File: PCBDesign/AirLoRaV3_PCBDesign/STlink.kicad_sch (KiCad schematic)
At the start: 1 part, among them J7 UART2

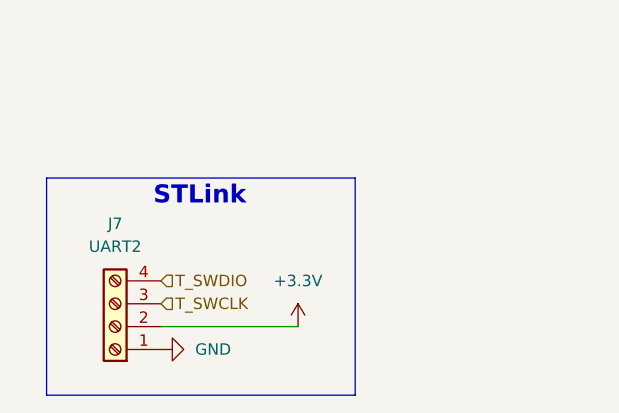
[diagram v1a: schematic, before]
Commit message: Update schematic
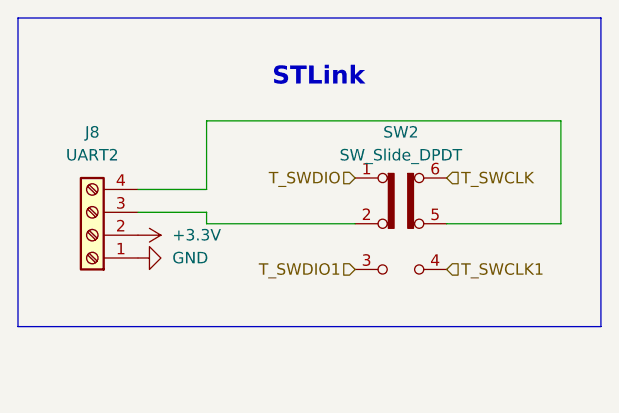
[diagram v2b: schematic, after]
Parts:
- added SW2: SW_Slide_DPDT, Button_Switch_THT:SW_E-Switch_EG1271_SPDT, symbol Switch:SW_Slide_DPDT
- renumbered J7 to J8
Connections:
- net T_SWCLK: now also SW2.6 (C); no longer J8.3 (Pin_3)
- net T_SWDIO: now also SW2.1 (A); no longer J8.4 (Pin_4)
- new net: J8.3 (Pin_3), SW2.2 (B)
- new net: J8.4 (Pin_4), SW2.5 (B)
- new net T_SWCLK1: SW2.4 (A)
- new net T_SWDIO1: SW2.3 (C)
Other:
- moved on the sheet: J8
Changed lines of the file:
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@@
 	(wire
 		(pts
-			(xy 142.24 100.33) (xy 157.48 100.33)
+			(xy 147.32 77.47) (xy 147.32 85.09)
+		)
+		(stroke
+			(width 0)
+			(type default)
+		)
+	)
+	(wire
+		(pts
+			(xy 147.32 85.09) (xy 139.7 85.09)
+		)
+		(stroke
+			(width 0)
+			(type default)
+		)
+	)
+	(wire
+		(pts
+			(xy 147.32 88.9) (xy 163.83 88.9)
+		)
+		(stroke
+			(width 0)
+			(type default)
+		)
+	)
+	(wire
+		(pts
+			(xy 147.32 87.63) (xy 139.7 87.63)
+		)
+		(stroke
+			(width 0)
+			(type default)
+		)
+	)
+	(wire
+		(pts
+			(xy 186.69 88.9) (xy 186.69 77.47)
+		)
+		(stroke
+			(width 0)
+			(type default)
+		)
+	)
+	(wire
+		(pts
+			(xy 186.69 77.47) (xy 147.32 77.47)
+		)
+		(stroke
+			(width 0)
+			(type default)
+		)
+	)
+	(wire
+		(pts
+			(xy 147.32 88.9) (xy 147.32 87.63)
+		)
+		(stroke
+			(width 0)
+			(type default)
+		)
+	)
+	(wire
+		(pts
+			(xy 173.99 88.9) (xy 186.69 88.9)
 		)
 		(stroke
@@
 	)
 	(rectangle
-		(start 129.54 83.82)
-		(end 163.83 107.95)
+		(start 126.365 66.04)
+		(end 191.135 100.33)
 		(stroke
 			(width 0)
@@
 	(text "STLink"
 		(exclude_from_sim no)
-		(at 146.558 85.852 0)
+		(at 159.766 72.644 0)
 		(effects
 			(font
@@
 		)
 	)
-	(hierarchical_label "T_SWCLK"
+	(hierarchical_label "T_SWCLK1"
 		(shape input)
-		(at 142.24 97.79 0)
+		(at 173.99 93.98 0)
 		(fields_autoplaced yes)
 		(effects
@@
 		)
 	)
-	(hierarchical_label "T_SWDIO"
+	(hierarchical_label "T_SWCLK"
 		(shape input)
-		(at 142.24 95.25 0)
+		(at 173.99 83.82 0)
 		(fields_autoplaced yes)
 		(effects
@@
 		)
 	)
+	(hierarchical_label "T_SWDIO"
+		(shape input)
+		(at 163.83 83.82 180)
+		(fields_autoplaced yes)
+		(effects
+			(font
+				(size 1.27 1.27)
+			)
+			(justify right)
+		)
+	)
+	(hierarchical_label "T_SWDIO1"
+		(shape input)
+		(at 163.83 93.98 180)
+		(fields_autoplaced yes)
+		(effects
+			(font
+				(size 1.27 1.27)
+			)
+			(justify right)
+		)
+	)
 	(symbol
 		(lib_id "Connector:Screw_Terminal_01x04")
-		(at 137.16 100.33 180)
+		(at 134.62 90.17 180)
 		(unit 1)
 		(exclude_from_sim no)
@@
 		(dnp no)
 		(fields_autoplaced yes)
-		(property "Reference" "J7"
-			(at 137.16 88.9 0)
+		(property "Reference" "J8"
+			(at 134.62 78.74 0)
 			(effects
 				(font
@@
 		)
 		(property "Value" "UART2"
-			(at 137.16 91.44 0)
+			(at 134.62 81.28 0)
 			(effects
 				(font
@@
 		)
 		(property "Footprint" "Connector_JST:JST_XH_B4B-XH-A_1x04_P2.50mm_Vertical"
-			(at 137.16 100.33 0)
+			(at 134.62 90.17 0)
 			(effects
 				(font
@@
 		)
 		(property "Datasheet" "~"
-			(at 137.16 100.33 0)
+			(at 134.62 90.17 0)
 			(effects
 				(font
@@
 		)
 		(property "Description" ""
-			(at 137.16 100.33 0)
+			(at 134.62 90.17 0)
 			(effects
 				(font
@@
 		)
 		(property "MANUFACTURER" ""
-			(at 137.16 100.33 0)
+			(at 134.62 90.17 0)
 			(effects
 				(font
@@
 		)
 		(property "MAXIMUM_PACKAGE_HEIGHT" ""
-			(at 137.16 100.33 0)
+			(at 134.62 90.17 0)
 			(effects
 				(font
@@
 		)
 		(property "PARTREV" ""
-			(at 137.16 100.33 0)
+			(at 134.62 90.17 0)
 			(effects
 				(font
@@
 		)
 		(property "STANDARD" ""
-			(at 137.16 100.33 0)
+			(at 134.62 90.17 0)
 			(effects
 				(font
@@
 			(project "airlora-kicad"
 				(path "/59d971df-d6c1-4ef7-a085-bf08b7b16047/be77b740-d58b-414b-97ce-61f1d1685314/0fe76900-3fef-41a8-aa6f-27268a6f6f64"
-					(reference "J7")
+					(reference "J8")
 					(unit 1)
 				)
@@
 	(symbol
 		(lib_id "power:GND")
-		(at 142.24 102.87 90)
+		(at 139.7 92.71 90)
 		(unit 1)
 		(exclude_from_sim no)
@@
 		(dnp no)
 		(fields_autoplaced yes)
-		(property "Reference" "#PWR043"
-			(at 148.59 102.87 0)
+		(property "Reference" "#PWR046"
+			(at 146.05 92.71 0)
 			(effects
 				(font
@@
 		)
 		(property "Value" "GND"
-			(at 146.05 102.8699 90)
+			(at 143.51 92.7099 90)
 			(effects
 				(font
@@
 		)
 		(property "Footprint" ""
-			(at 142.24 102.87 0)
+			(at 139.7 92.71 0)
 			(effects
 				(font
@@
 		)
 		(property "Datasheet" ""
-			(at 142.24 102.87 0)
+			(at 139.7 92.71 0)
 			(effects
 				(font
@@
 		)
 		(property "Description" "Power symbol creates a global label with name \"GND\" , ground"
-			(at 142.24 102.87 0)
+			(at 139.7 92.71 0)
 			(effects
 				(font
@@
 			(project "airlora-kicad"
 				(path "/59d971df-d6c1-4ef7-a085-bf08b7b16047/be77b740-d58b-414b-97ce-61f1d1685314/0fe76900-3fef-41a8-aa6f-27268a6f6f64"
-					(reference "#PWR043")
+					(reference "#PWR046")
 					(unit 1)
 				)
@@
 	(symbol
 		(lib_id "power:+3.3V")
-		(at 157.48 100.33 0)
+		(at 139.7 90.17 270)
 		(unit 1)
 		(exclude_from_sim no)
@@
 		(dnp no)
 		(fields_autoplaced yes)
-		(property "Reference" "#PWR044"
-			(at 157.48 104.14 0)
+		(property "Reference" "#PWR045"
+			(at 135.89 90.17 0)
 			(effects
 				(font
@@
 		)
 		(property "Value" "+3.3V"
-			(at 157.48 95.25 0)
-			(effects
-				(font
-					(size 1.27 1.27)
-				)
+			(at 143.51 90.1699 90)
+			(effects
+				(font
+					(size 1.27 1.27)
+				)
+				(justify left)
 			)
 		)
 		(property "Footprint" ""
-			(at 157.48 100.33 0)
+			(at 139.7 90.17 0)
 			(effects
 				(font
@@
 		)
 		(property "Datasheet" ""
-			(at 157.48 100.33 0)
+			(at 139.7 90.17 0)
 			(effects
 				(font
@@
 		)
 		(property "Description" "Power symbol creates a global label with name \"+3.3V\""
-			(at 157.48 100.33 0)
+			(at 139.7 90.17 0)
 			(effects
 				(font
@@
 			(project "airlora-kicad"
 				(path "/59d971df-d6c1-4ef7-a085-bf08b7b16047/be77b740-d58b-414b-97ce-61f1d1685314/0fe76900-3fef-41a8-aa6f-27268a6f6f64"
-					(reference "#PWR044")
+					(reference "#PWR045")
 					(unit 1)
 				)
+			)
+		)
+	)
+	(symbol
+		(lib_id "Switch:SW_Slide_DPDT")
+		(at 168.91 88.9 0)
+		(unit 1)
+		(exclude_from_sim no)
+		(in_bom yes)
+		(on_board yes)
+		(dnp no)
+		(fields_autoplaced yes)
+		(property "Reference" "SW2"
+			(at 168.91 78.74 0)
+			(effects
+				(font
+					(size 1.27 1.27)
+				)
+			)
+		)
+		(property "Value" "SW_Slide_DPDT"
+			(at 168.91 81.28 0)
+			(effects
+				(font
+					(size 1.27 1.27)
+				)
+			)
+		)
+		(property "Footprint" "Button_Switch_THT:SW_E-Switch_EG1271_SPDT"
+			(at 182.88 83.82 0)
+			(effects
+				(font
+					(size 1.27 1.27)
+				)
+				(hide yes)
+			)
+		)
+		(property "Datasheet" "~"
+			(at 168.91 88.9 0)
+			(effects
+				(font
+					(size 1.27 1.27)
+				)
+				(hide yes)
+			)
+		)
+		(property "Description" "Slide Switch, dual pole double throw"
+			(at 168.91 88.9 0)
+			(effects
+				(font
+					(size 1.27 1.27)
+				)
+				(hide yes)
+			)
+		)
+		(pin "6"
+		)
+		(pin "4"
+		)
+		(pin "1"
+		)
+		(pin "3"
+		)
+		(pin "5"
+		)
+		(pin "2"
+		)
+		(instances
+			(project "airlora-kicad"
+				(path "/59d971df-d6c1-4ef7-a085-bf08b7b16047/be77b740-d58b-414b-97ce-61f1d1685314/0fe76900-3fef-41a8-aa6f-27268a6f6f64"
+					(reference "SW2")
+					(unit 1)
+				)
